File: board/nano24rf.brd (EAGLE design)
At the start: 17.4 x 50 mm, 18 parts

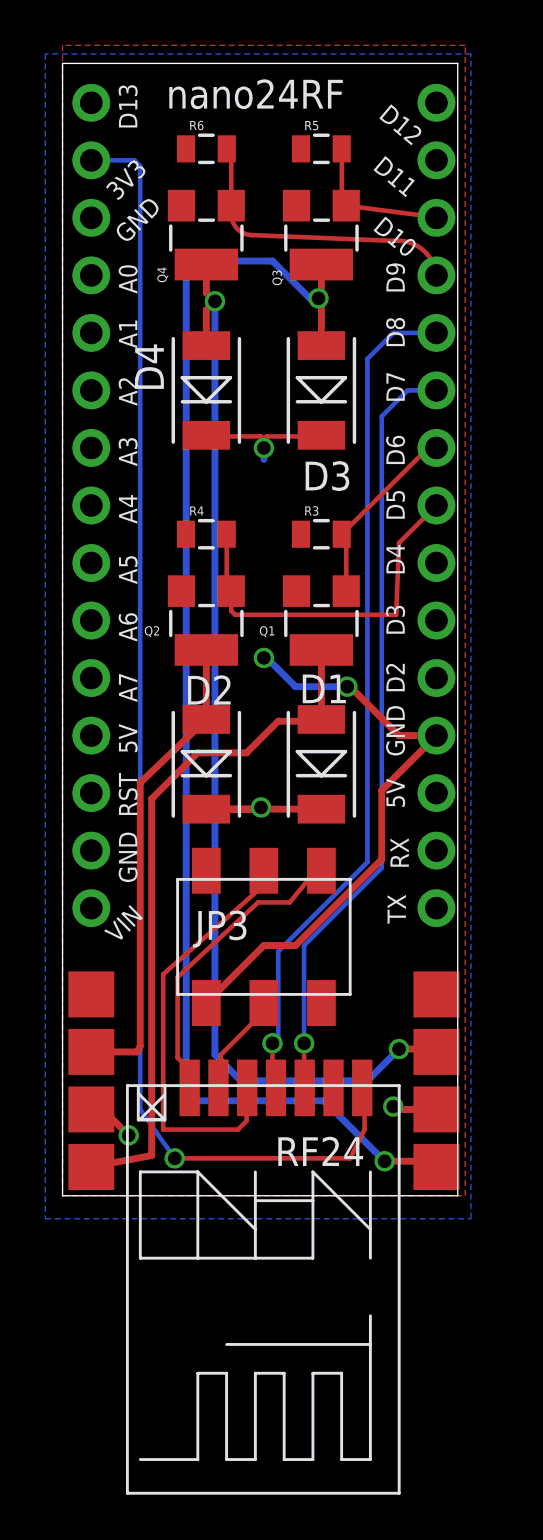
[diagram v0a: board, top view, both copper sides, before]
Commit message: added gerber for cestlation fike
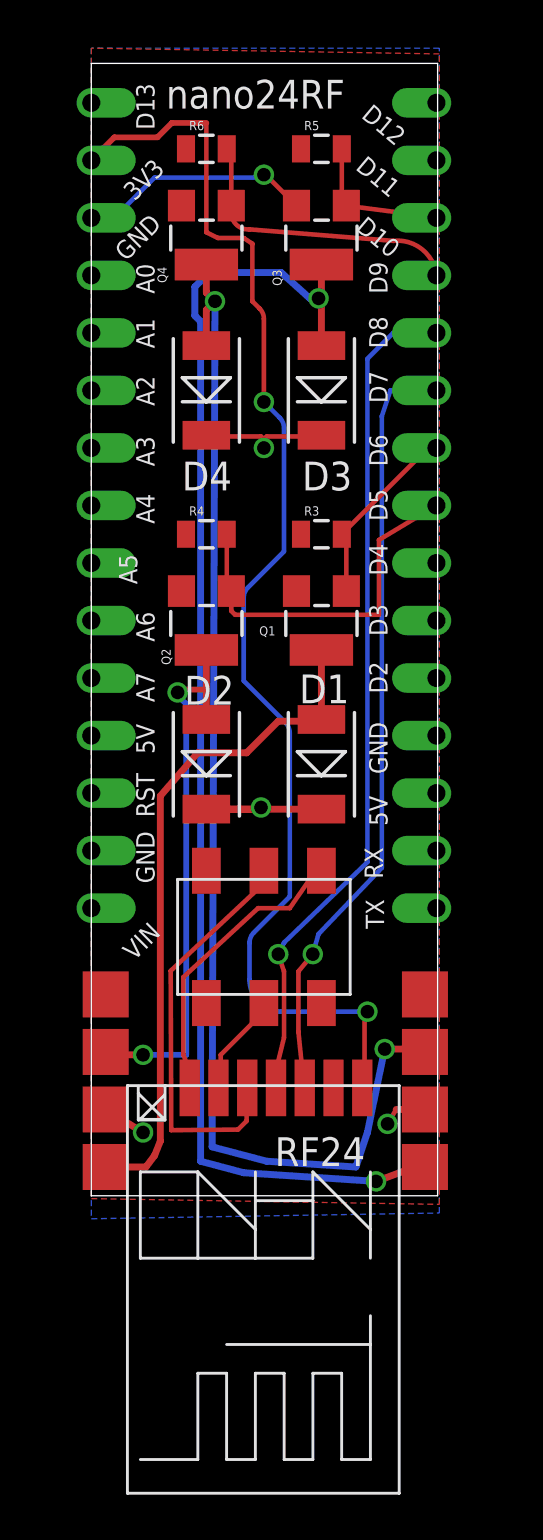
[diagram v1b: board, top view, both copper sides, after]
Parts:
- JP1, JP2: device microbuilder:1X15_ROUND_70 -> nano24rf:1X15_LONG
- moved MOSFET-12 0.64 mm to (1.91, 5.08)
- moved MOSFET-34 0.51 mm to (16.0, 5.08)
- flipped JP1 to the bottom
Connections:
- net 3V3: now also JP1.P$2; no longer JP1.2
- net CE: now also JP2.P$6; no longer JP2.6
- net CSN: now also JP2.P$5; no longer JP2.5
- net D10: now also JP2.P$3; no longer JP2.3
- net D5: now also JP2.P$8; no longer JP2.8
- net D6: now also JP2.P$7; no longer JP2.7
- net D9: now also JP2.P$4; no longer JP2.4
- net GND: now also JP1.P$14, JP1.P$3, JP2.P$12; no longer JP1.14, JP1.3, JP2.12
- net SCL: now also JP1.P$9; no longer JP1.9
- net SDA: now also JP1.P$8; no longer JP1.8
- net VIN: now also JP1.P$15; no longer JP1.15
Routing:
- net GND: track 26.3 -> 10.3 mm, vias 2 -> 1
- net FET04: track 48.1 -> 55.6 mm
- net FET02: track 21.1 -> 24.2 mm, vias 0 -> 2
- net 3V3: track 57.6 -> 59.3 mm, vias 1 -> 2
- net VIN: track 18.4 -> 17.5 mm
- net CSK: track 18.7 -> 18.2 mm
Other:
- board size 17.4 x 50 mm -> 15.3 x 50 mm

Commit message: back to round ads
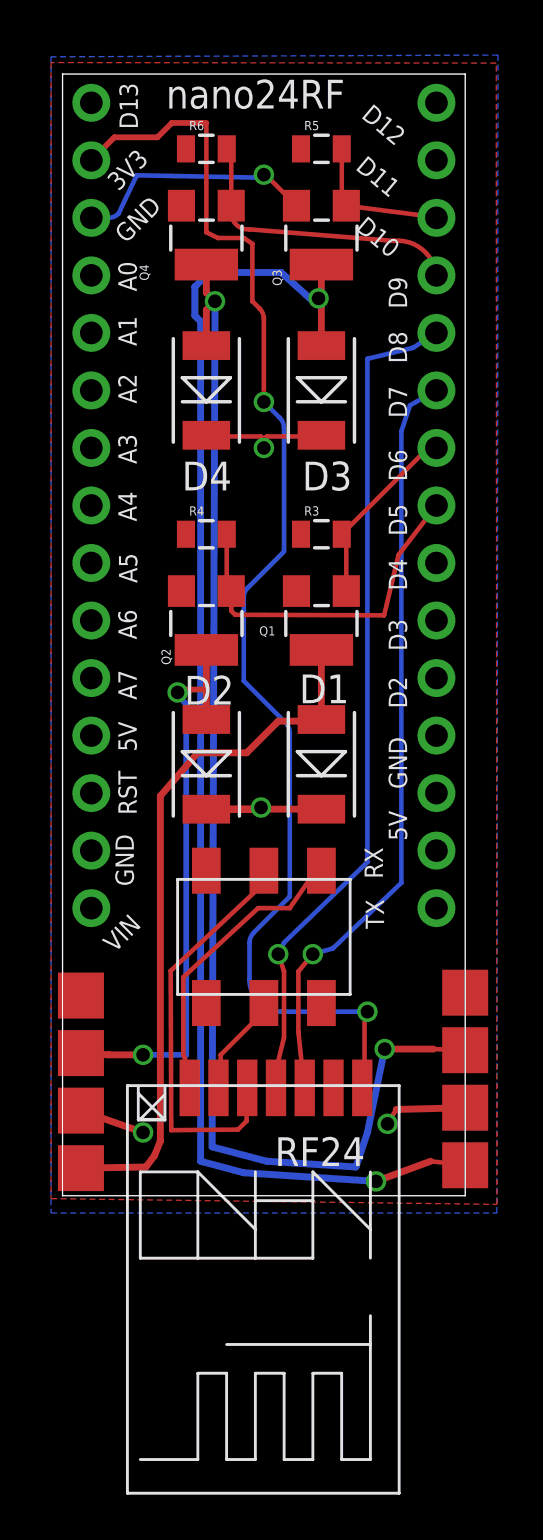
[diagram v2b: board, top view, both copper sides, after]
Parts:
- JP1, JP2: device nano24rf:1X15_LONG -> nano24rf:1X15_ROUND_70
- moved MOSFET-34 1.78 mm to (17.8, 5.16)
- moved MOSFET-12 1.09 mm to (0.81, 5.03)
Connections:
- net 3V3: now also JP1.2; no longer JP1.P$2
- net CE: now also JP2.6; no longer JP2.P$6
- net CSN: now also JP2.5; no longer JP2.P$5
- net D10: now also JP2.3; no longer JP2.P$3
- net D5: now also JP2.8; no longer JP2.P$8
- net D6: now also JP2.7; no longer JP2.P$7
- net D9: now also JP2.4; no longer JP2.P$4
- net GND: now also JP1.14, JP1.3, JP2.12; no longer JP1.P$14, JP1.P$3, JP2.P$12
- net SCL: now also JP1.9; no longer JP1.P$9
- net SDA: now also JP1.8; no longer JP1.P$8
- net VIN: now also JP1.15; no longer JP1.P$15
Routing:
- net VIN: track 17.5 -> 20.2 mm
- net FET03: track 59.5 -> 60.7 mm
- net FET01: track 30.0 -> 31.1 mm
- net FET02: track 24.2 -> 25.2 mm
- net FET04: track 55.6 -> 56.6 mm
- net CE: track 34.3 -> 33.8 mm
- net D5: track 16.3 -> 15.8 mm
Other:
- board size 15.3 x 50 mm -> 17.8 x 49.5 mm
